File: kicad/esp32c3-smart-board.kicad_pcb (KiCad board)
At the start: 4 copper layers, 38.1 x 43.1 mm, 69 parts, among them J1 USB_C_Receptacle_USB2.0_16P, J3 Conn_01x12_Pin, Q1 FS8205A, Q2 BSS138, Q3 IRLML6401, SW1 SW_Push, SW2 SW_Push, U1 ME6211C33M5G, U2 ESP32-C3, U3 TP4056, U4 MPU-6050, U5 DW01A, Y1 SJK-7U-40.000

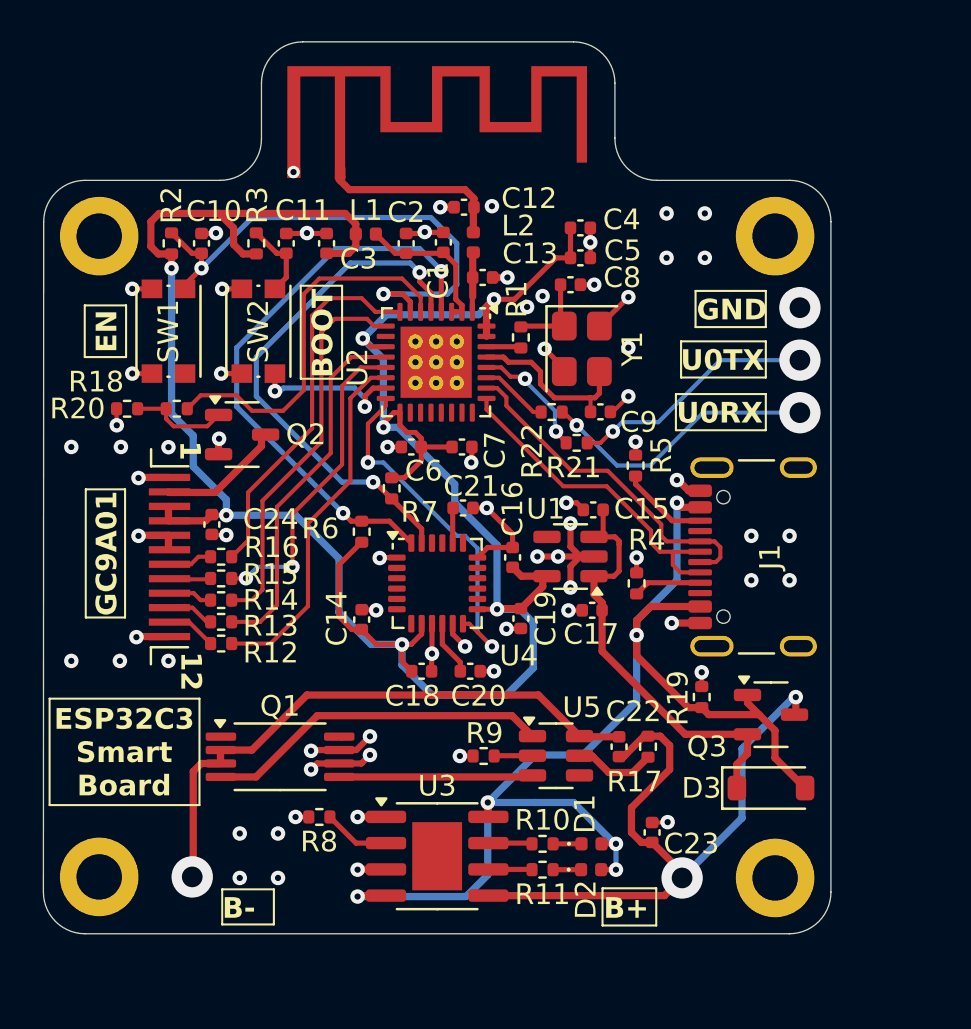
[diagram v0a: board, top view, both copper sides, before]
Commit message: Update KiCAD project for revision 1.3
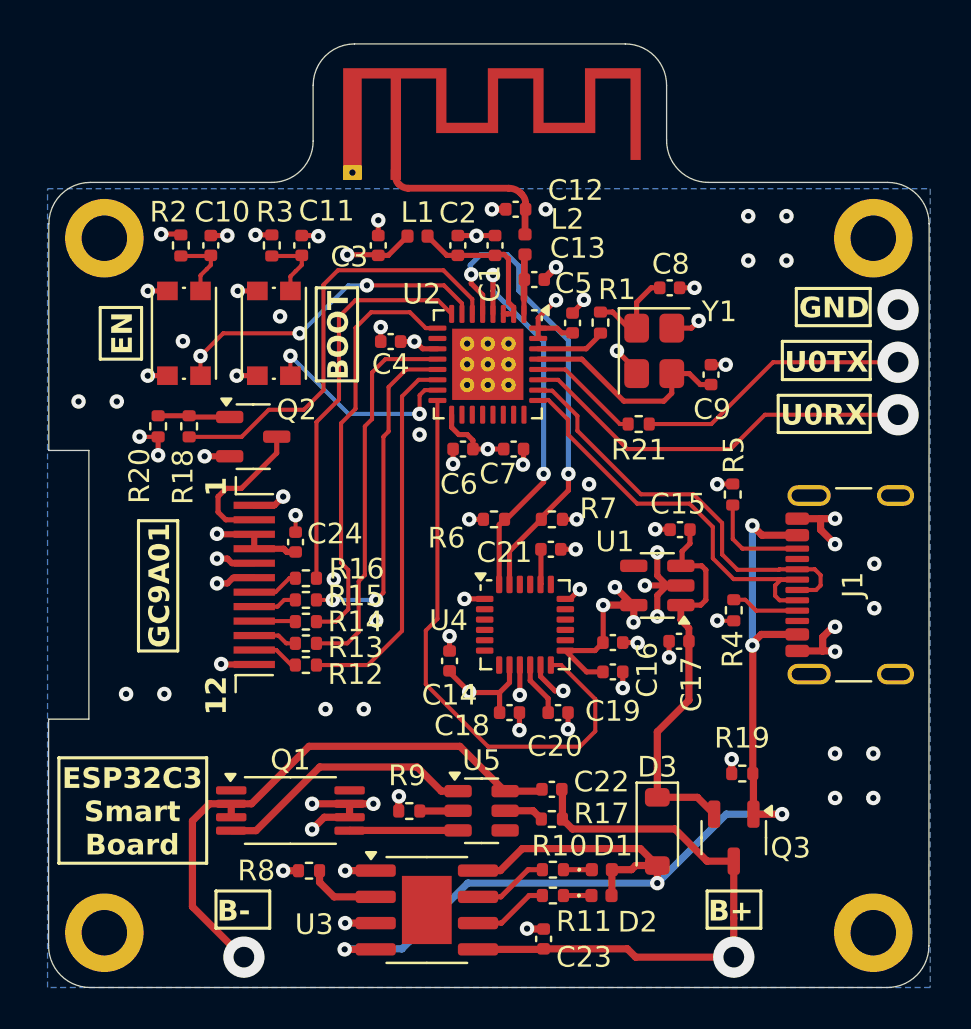
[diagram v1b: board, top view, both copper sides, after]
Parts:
- removed R22: 100R, Resistor_SMD:R_0402_1005Metric
- AE1: footprint User:ESPRESSIF_ESP32_MIFA_2.4GHz_Right -> RF_Antenna:Texas_SWRA117D_2.4GHz_Right
- moved C4 10.7 mm to (28.9, 26.6), turned to 180 degrees
- moved R7 7.89 mm to (36.6, 35.2), turned to 0 degrees
- moved C23 7.35 mm to (36.2, 55.5)
- moved R6 6.43 mm to (33.9, 35.2), turned to 0 degrees
- moved C16 6.36 mm to (39.6, 41.2), turned to 0 degrees
- moved Q3 6.22 mm to (45.5, 50.6), turned to -90 degrees
- moved D3 5.89 mm to (41.8, 50.3), turned to -90 degrees
- moved R17 5.82 mm to (36.6, 49.7), turned to 0 degrees
- moved C9 5.64 mm to (44.4, 28.2), turned to 90 degrees
- moved H3 5.44 mm to (52.2, 55.2)
- moved C19 5.14 mm to (39.6, 42.6), turned to 0 degrees
- moved R5 4.90 mm to (45.4, 34.0)
- moved J1 4.89 mm to (52.2, 38.4)
- moved R4 4.88 mm to (45.5, 39.6), turned to -90 degrees
- moved C8 4.80 mm to (42.4, 24.0)
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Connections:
- U2 pad 27: Net-(U2-U0RXD/GPIO20) -> /U0RX
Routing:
- net +3.3V: track 118.2 -> 36.2 mm, vias 7 -> 13
- net /MPU_INT: track 17.4 -> 28.1 mm, vias 2 -> 0
- net /I2C_SDA: track 28.4 -> 18.9 mm
- net /CHIP_EN: track 26.6 -> 19.4 mm, vias 2 -> 3
- net +BATT: track 33.3 -> 27.8 mm, vias 2 -> 1
- net /U0RX: track 13.6 -> 18.5 mm, vias 2 -> 1
- net /D-: track 16.2 -> 20.3 mm
- net Net-(U5-OC): track 9.36 -> 5.26 mm
- net /D+: track 16.4 -> 20.4 mm
- net Net-(U5-OD): track 16.7 -> 12.7 mm
- net Net-(U2-U0RXD/GPIO20): track 3.33 -> 0.00 mm
- net /BL: track 18.3 -> 21.3 mm
- net /I2C_SCL: track 25.6 -> 23.1 mm
- net /BOOT: track 11.4 -> 13.7 mm
- net GND: track 63.4 -> 65.6 mm, vias 73 -> 80
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- added copper zone on B.Cu, net +3.3V
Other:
- board size 38.1 x 43.1 mm -> 42.6 x 45.7 mm
